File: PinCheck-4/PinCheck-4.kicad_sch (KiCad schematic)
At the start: 0 parts

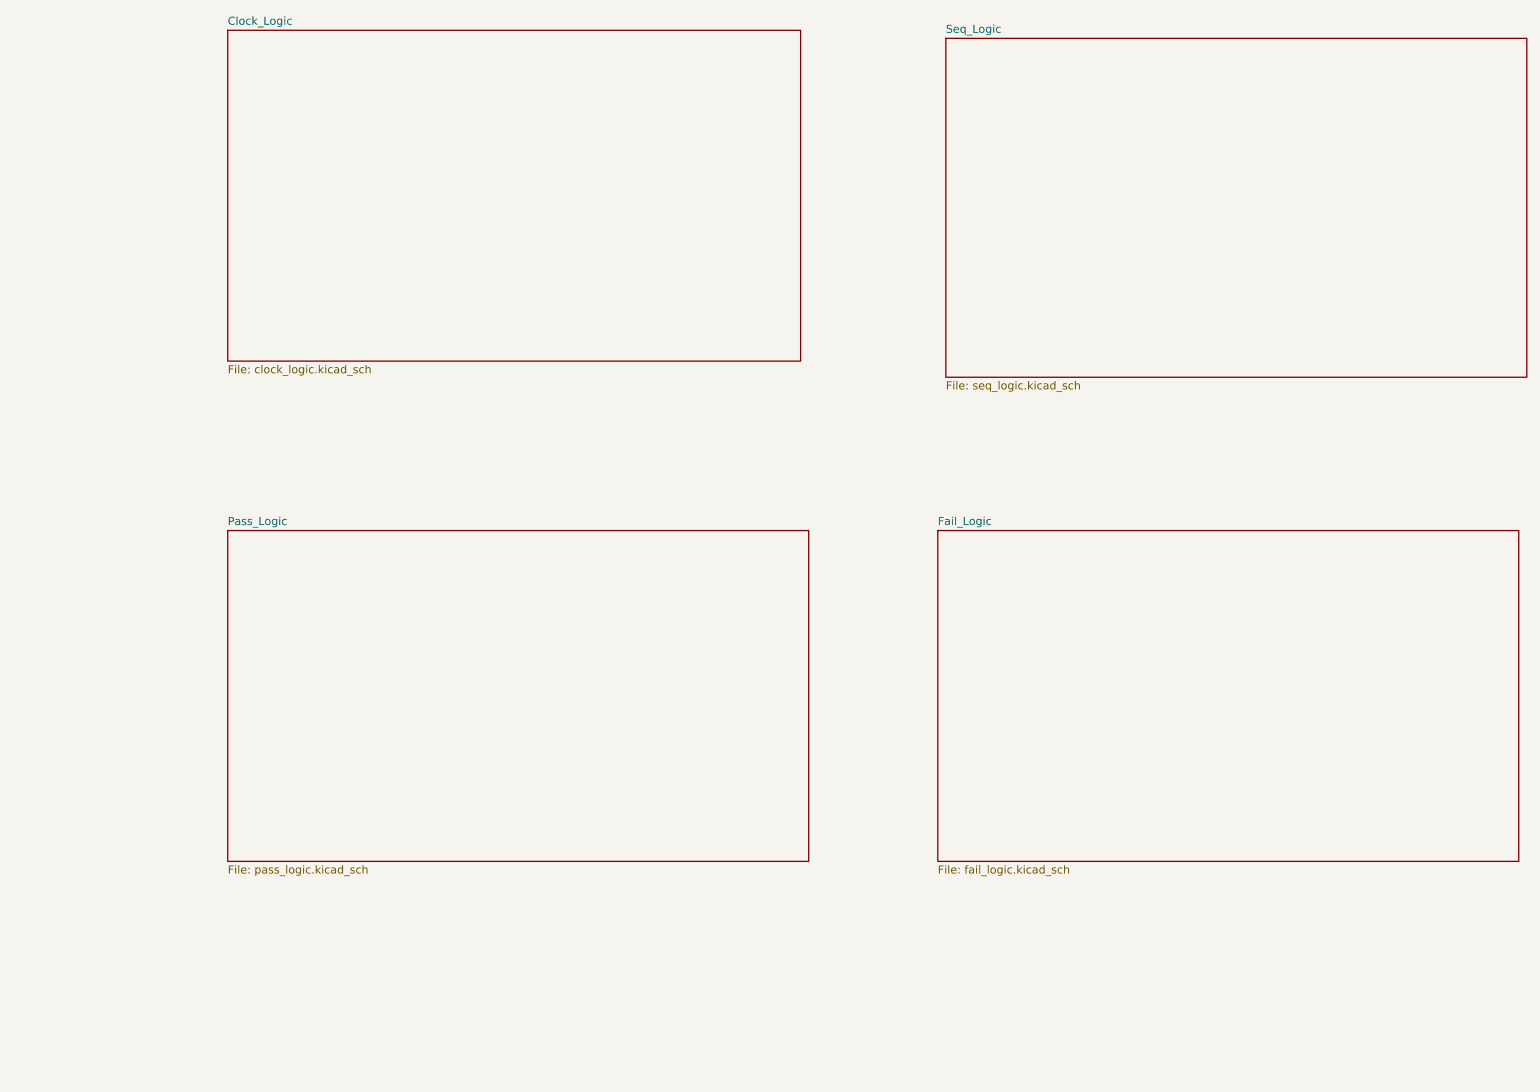
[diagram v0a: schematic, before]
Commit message: Daily sync 2025-08-27 16:57
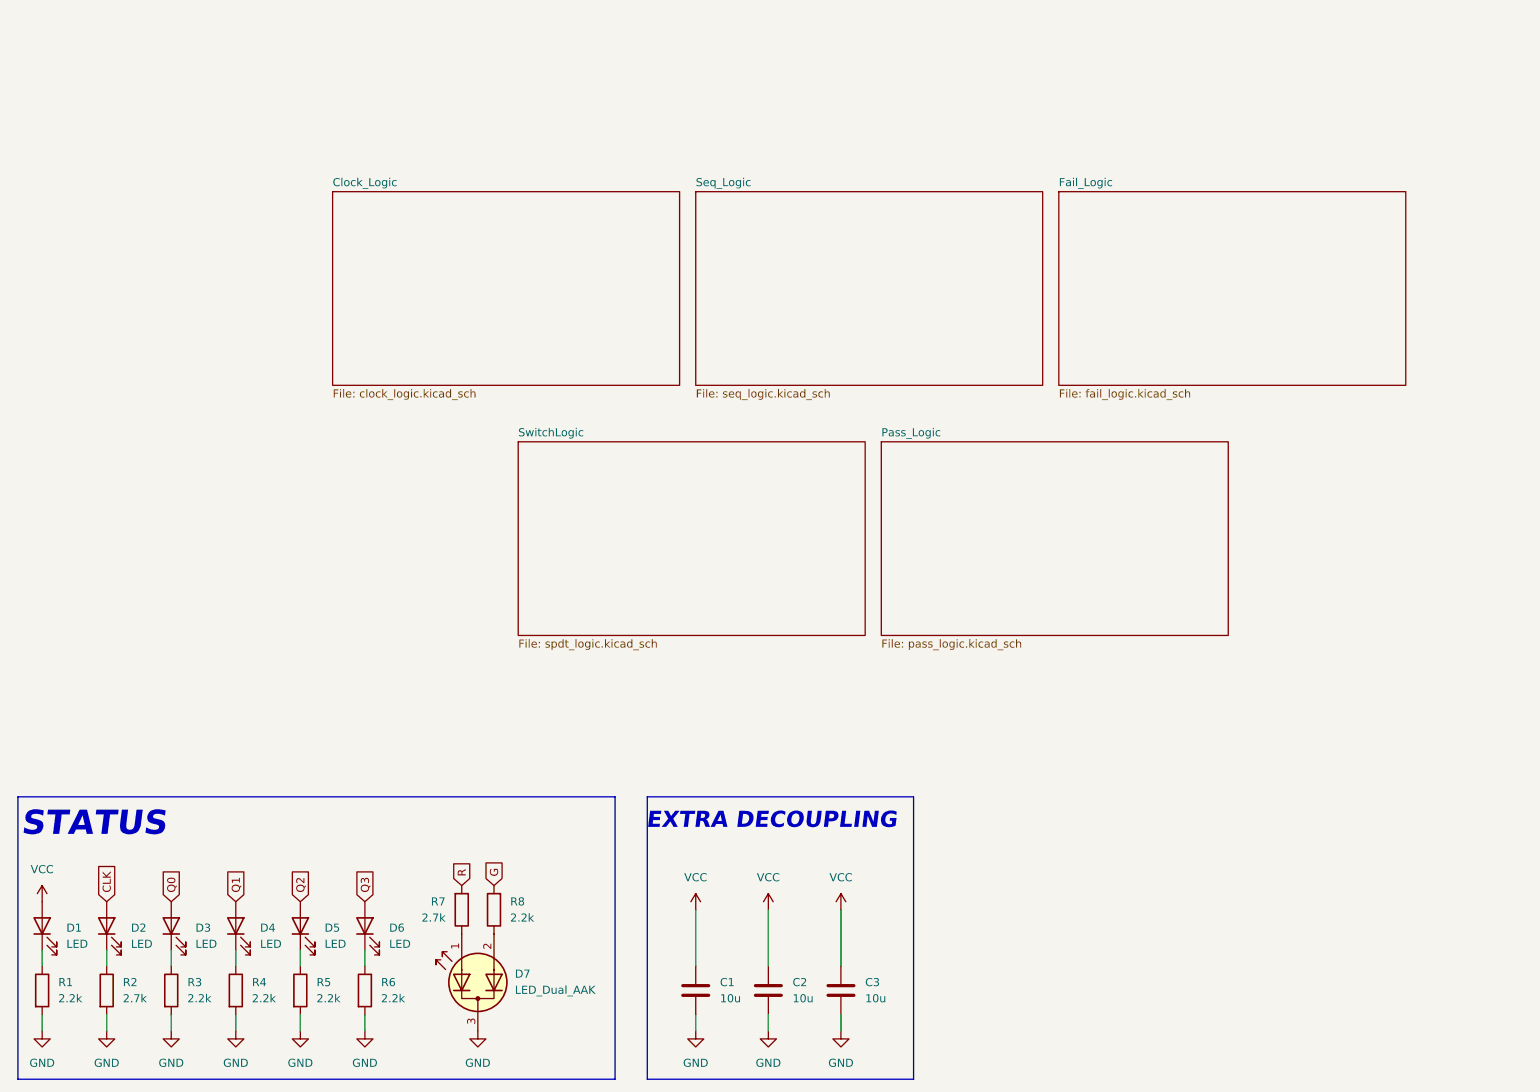
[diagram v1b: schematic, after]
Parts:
- added C1, C2, C3: 10u, Capacitor_SMD:C_0805_2012Metric, symbol Device:C
- added D1, D2, D3, D4, D5, D6: LED, LED_THT:LED_D3.0mm_Clear, symbol Device:LED
- added D7: LED_Dual_AAK, LED_THT:LED_D3.0mm-3, symbol Device:LED_Dual_AAK
- added R1, R3, R4, R5, R6, R8: 2.2k, Resistor_SMD:R_0805_2012Metric, symbol Device:R
- added R2, R7: 2.7k, Resistor_SMD:R_0805_2012Metric, symbol Device:R
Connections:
- new net: D1.1 (K), R1.1
- new net: D6.1 (K), R6.1
- new net: D5.1 (K), R5.1
- new net: D4.1 (K), R4.1
- new net: D7.1 (A1), R7.1
- new net: D7.2 (A2), R8.1
- new net: D3.1 (K), R3.1
- new net: D2.1 (K), R2.1
- new net CLK: D2.2 (A)
- new net G: R8.2
- new net GND: C1.2, C2.2, C3.2, D7.3 (K), R1.2, R2.2, R3.2, R4.2, R5.2, R6.2
- new net Q0: D3.2 (A)
- new net Q1: D4.2 (A)
- new net Q2: D5.2 (A)
- new net Q3: D6.2 (A)
- new net R: R7.2
- new net VCC: C1.1, C2.1, C3.1, D1.2 (A)
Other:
- added sheet SwitchLogic (spdt_logic.kicad_sch)
- note added: "EXTRA DECOUPLING"
- note added: "STATUS"
